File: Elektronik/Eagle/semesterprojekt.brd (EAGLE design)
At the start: 84.8 x 80 mm, 37 parts, among them T1 BC457, T2 BC457, T3 BC457, T5 BC457, T6 BC457, T7 BC457, X1 22-23-2041

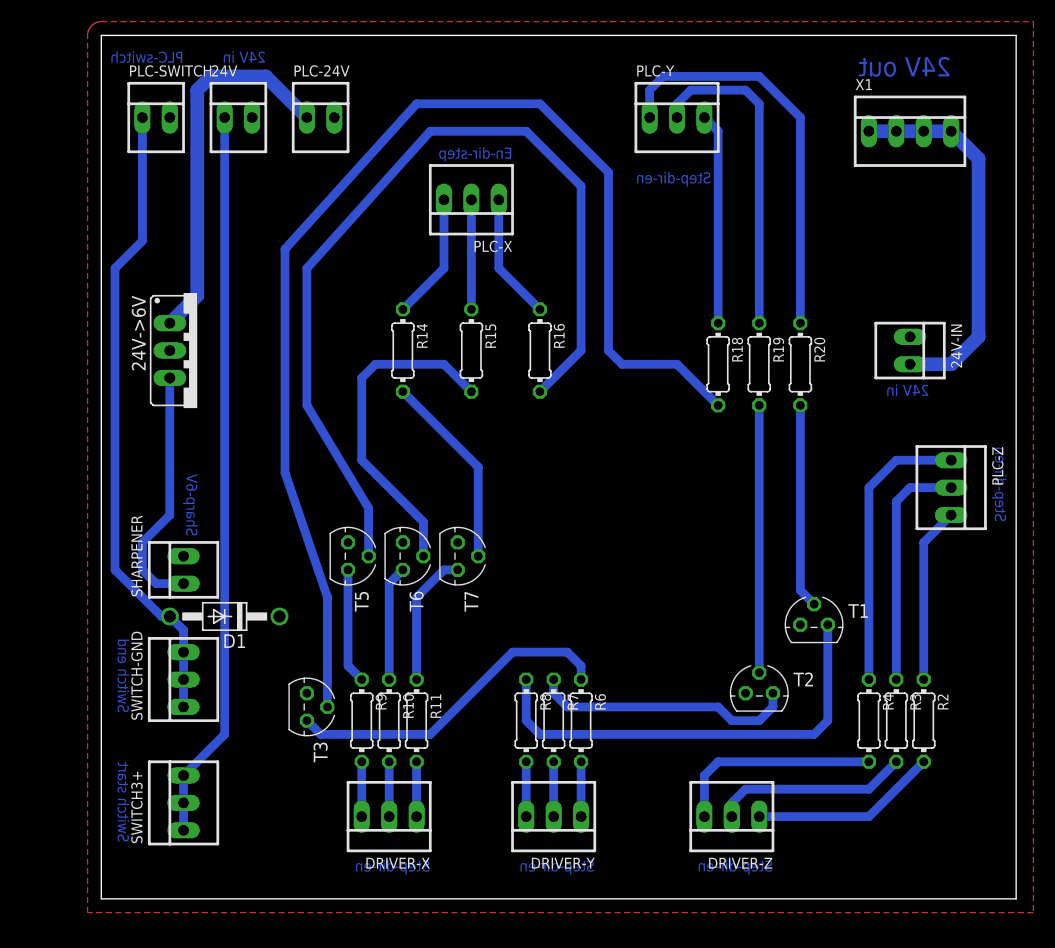
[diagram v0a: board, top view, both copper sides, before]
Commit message: boardv4
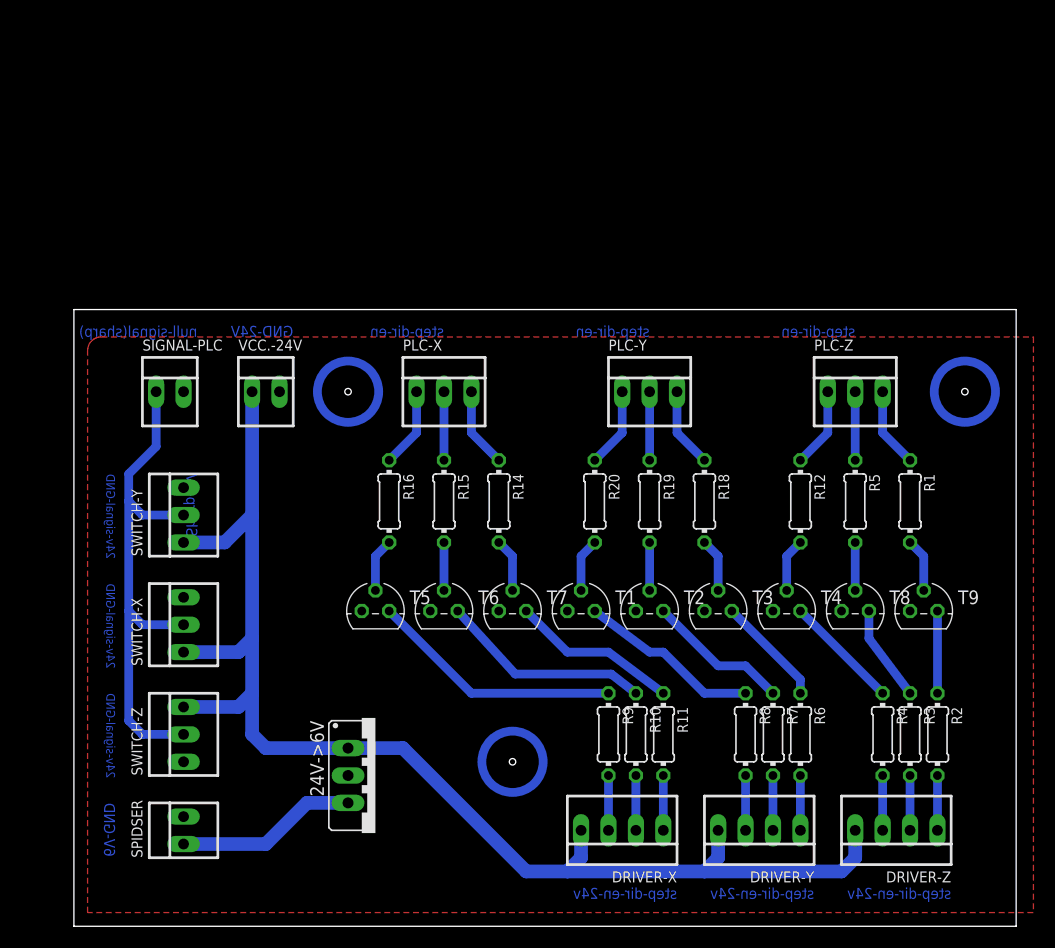
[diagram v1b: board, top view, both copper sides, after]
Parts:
- removed 24V, 24V-IN, PLC-24V, PLC-SWITCH, SHARPENER: 22-23-2021, con-molex:22-23-2021
- removed D1: 1N4004, diode:DO41-10
- removed SWITCH-GND, SWITCH3+: 22-23-2031, con-molex:22-23-2031
- removed X1: 22-23-2041, con-molex:22-23-2041
- added R1, R12, R5: 5K, rcl:0204/7
- added SIGNAL-PLC, SPIDSER, VCC.-24V: 22-23-2021, con-molex:22-23-2021
- added SWITCH-X, SWITCH-Y, SWITCH-Z: 22-23-2031, con-molex:22-23-2031
- added T4, T8, T9: BC547, transistor:TO92
- DRIVER-X, DRIVER-Y, DRIVER-Z: value 22-23-2031 -> 22-23-2041; device con-molex:22-23-2031 -> con-molex:22-23-2041
- T1, T2, T3, T5, T6, T7: value BC457 -> BC547
- moved 24V->6V 42.7 mm to (25.4, 11.4)
- moved T3 39.1 mm to (57.1, 26.7), turned to 0 degrees
- moved PLC-Y 25.5 mm to (50.8, 47.0)
- moved R20 22.9 mm to (45.7, 36.8)
- moved R9 22.9 mm to (47.0, 15.2)
- moved R10 22.9 mm to (49.5, 15.2)
- moved R11 22.9 mm to (52.1, 15.2)
- moved T1 21.6 mm to (44.5, 26.7)
- moved DRIVER-X 21.6 mm to (48.3, 6.35)
- moved R7 20.4 mm to (62.2, 15.2)
- moved R8 20.4 mm to (59.7, 15.2)
- moved R6 20.4 mm to (64.8, 15.2)
- moved R16 19.8 mm to (26.7, 36.8)
- moved DRIVER-Y 19.1 mm to (61.0, 6.35)
- moved PLC-X 18.0 mm to (31.8, 47.0), turned to 0 degrees
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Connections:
- removed net N$1: 24V-IN.2, X1.1, X1.2, X1.3, X1.4
- removed net N$13: 24V->6V.IN, PLC-24V.1
- new net N$16: SIGNAL-PLC.1, SWITCH-X.2, SWITCH-Y.2, SWITCH-Z.2
- new net N$30: R3.1, T8.1
- new net N$38: R12.2, T4.2
- new net N$39: R5.2, T8.2
- new net N$40: R1.2, T9.2
- new net VCC: 24V->6V.IN, DRIVER-X.4, DRIVER-Y.4, DRIVER-Z.4, SWITCH-X.1, SWITCH-Y.1, SWITCH-Z.3, VCC.-24V.1
- net GND: now also SPIDSER.2, SWITCH-X.3, SWITCH-Y.3, SWITCH-Z.1, T4.3, T8.3, T9.3, VCC.-24V.2; no longer 24V-IN.1, D1.C, PLC-24V.2, SHARPENER.2
- net N$14: now also R4.1, T4.1; no longer 24V->6V.OUT, SHARPENER.1
- net N$33: now also R2.1, T9.1; no longer PLC-Z.1, R4.1
- net N$34: now also PLC-Z.1, R12.1; no longer PLC-Z.2, R3.1
- net N$35: now also PLC-Z.2, R5.1; no longer PLC-Z.3, R2.1
- net N$36: now also PLC-Z.3, R1.1; no longer 24V.1, SWITCH3+.1, SWITCH3+.2, SWITCH3+.3
- net N$5: now also 24V->6V.OUT, SPIDSER.1; no longer D1.A, PLC-SWITCH.1, SWITCH-GND.1, SWITCH-GND.2, SWITCH-GND.3
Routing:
- net VCC: track 0.00 -> 125.8 mm
- net N$10: track 110.4 -> 4.97 mm
- net N$8: track 82.0 -> 4.97 mm
- net N$36: track 67.6 -> 7.40 mm
- net N$16: track 0.00 -> 48.4 mm
- net N$5: track 58.7 -> 16.8 mm
- net N$1: track 35.1 -> 0.00 mm
- net N$13: track 34.9 -> 0.00 mm
- net N$29: track 37.7 -> 7.40 mm
- net N$7: track 30.6 -> 4.45 mm
- net N$18: track 41.7 -> 16.8 mm
- net N$24: track 30.3 -> 6.35 mm
- net N$22: track 30.9 -> 10.3 mm
- net N$11: track 24.8 -> 4.45 mm
- net N$33: track 26.5 -> 7.62 mm
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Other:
- board size 84.8 x 80 mm -> 87.3 x 57.1 mm
- board text added: "24v-signal-GND"
- board text added: "6V-GND"
- board text added: "GND-24V"
- board text added: "null-signal(sharp)"
- board text added: "step-dir-en"
- board text added: "step-dir-en-24v"
- board text removed: "24V in"
- board text removed: "24V out"
- board text removed: "En-dir-step"
- board text removed: "PLC-switch"
- board text removed: "Step-dir-en"
- board text removed: "Switch end"
- board text removed: "Switch start"
